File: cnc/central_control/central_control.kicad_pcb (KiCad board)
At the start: 4 copper layers, 103 x 107 mm, 164 parts, among them J1 6pins, J10 Phoenix, J11 3pins, J12 3pins, J13 Screw_Terminal_01x01, J14 3pins, J16 Phoenix, J17 DE9_Socket_MountingHoles, J2 6pins, J20 AVR-UPDI, J3 6pins, J4 7pins, J5 7pins, J6 3pins, J7 3pins, J8 Phoenix, J9 Phoenix, U1 LMR33630ADDA, U10 PC817, U11 PCA9555PW, U12 PCA9555PW, U13 PCA9555PW, U14 PC817, U15 PC817, U16 PC817, U17 PC817, U18 PC817, U19 PC817, U2 LT1785AxS8, U3 ATtiny3226, U5 PC817, U6 PC817, U7 PC817, U8 PC817, U9 PC817

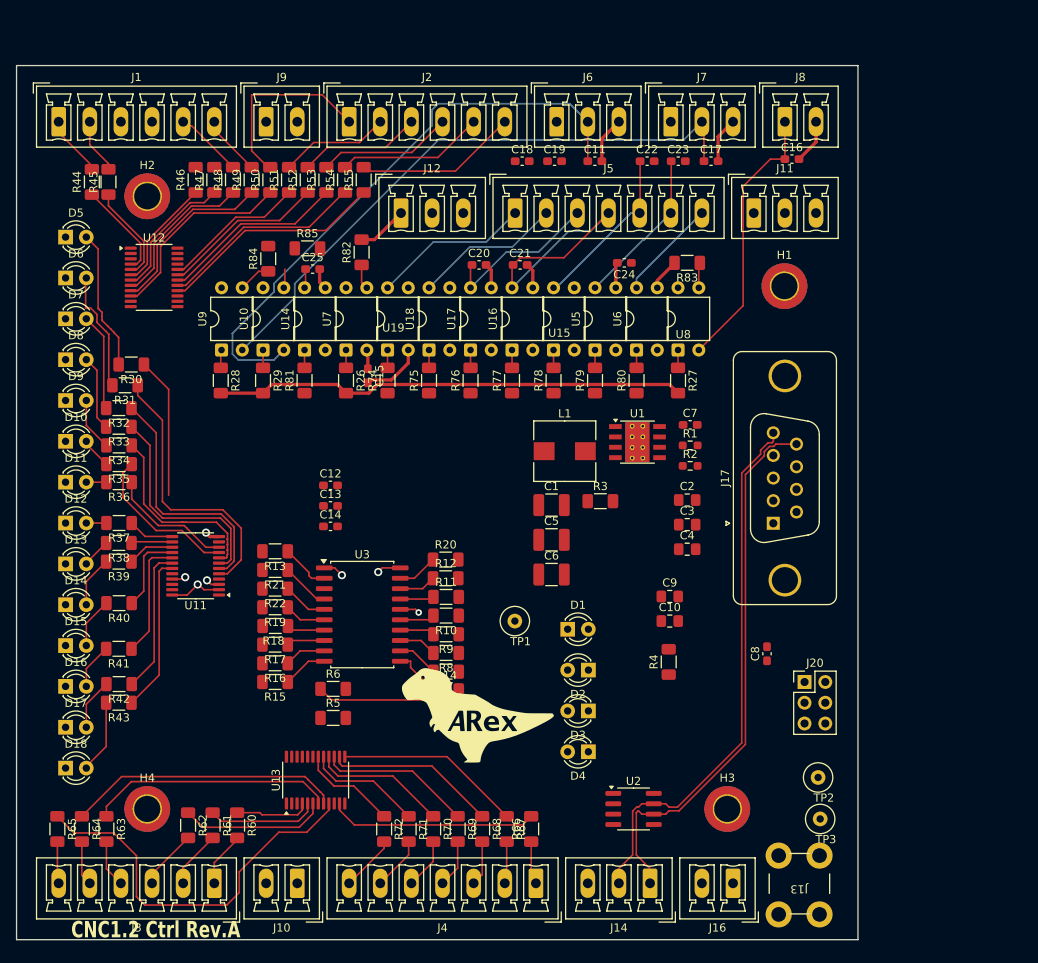
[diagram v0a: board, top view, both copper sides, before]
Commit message: Sent to production
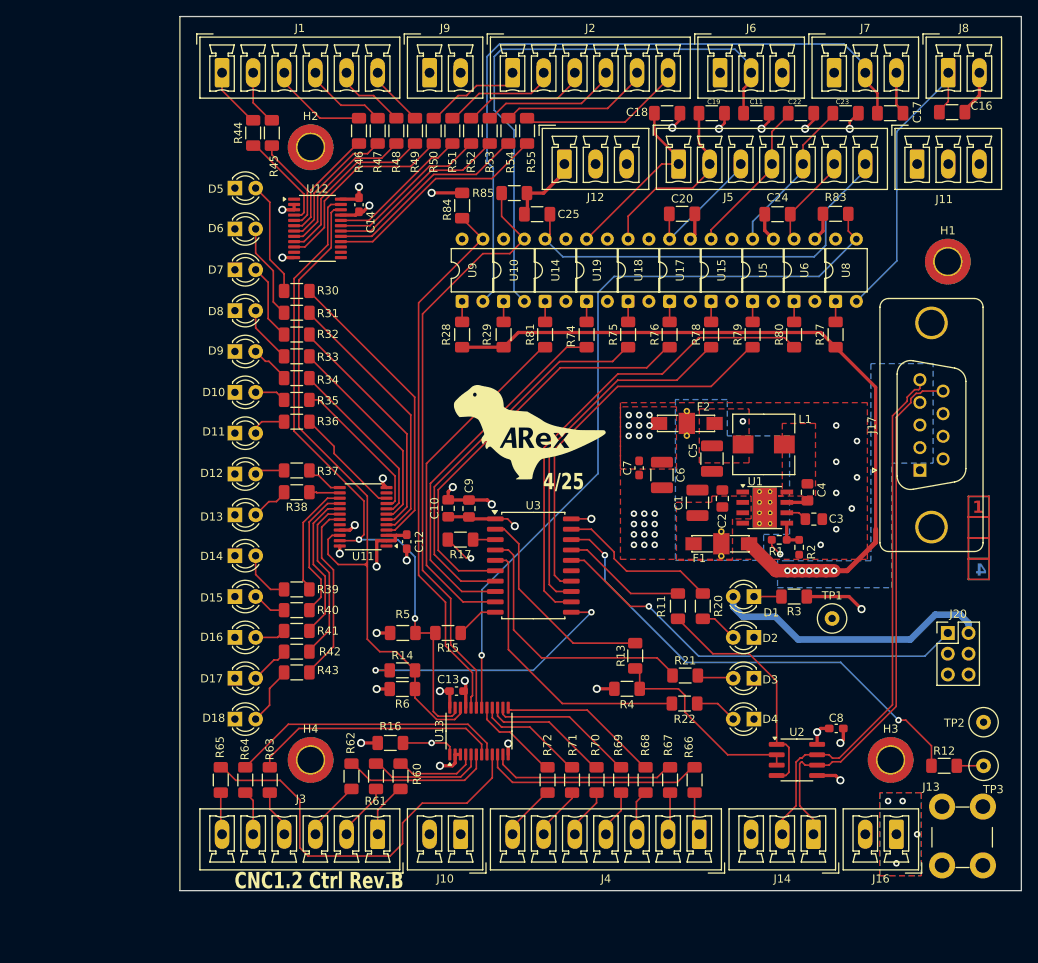
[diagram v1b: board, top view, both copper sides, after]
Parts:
- removed C15, C21: 1nF 250V, Capacitor_SMD:C_0603_1608Metric_Pad1.08x0.95mm_HandSolder
- removed R10, R18, R19, R7, R8, R9: 332, Resistor_SMD:R_1206_3216Metric_Pad1.30x1.75mm_HandSolder
- removed R26: 3k32, Resistor_SMD:R_1206_3216Metric_Pad1.30x1.75mm_HandSolder
- removed R77: 560, Resistor_SMD:R_1206_3216Metric_Pad1.30x1.75mm_HandSolder
- removed R82: 10K, Resistor_SMD:R_1206_3216Metric_Pad1.30x1.75mm_HandSolder
- removed U16, U7: PC817, Package_DIP:DIP-4_W7.62mm
- added F1: ~, adarwoo:Murata_NFM61R, F.Cu at (186.3, 107.5)
- added F2: ~, adarwoo:Murata_NFM61R, F.Cu at (182.1, 92.8)
- C11, C16, C17, C18, C19, C20, C22, C23, C24, C25: footprint Capacitor_SMD:C_0603_1608Metric_Pad1.08x0.95mm_HandSolder -> Capacitor_SMD:C_1206_3216Metric_Pad1.33x1.80mm_HandSolder
- J13: value Screw_Terminal_01x01 -> ~
- R16: value 332 -> 10K
- R27, R28, R29: value 3k32 -> 2k21
- moved R12 65.2 mm to (213.5, 134.7)
- moved R22 52.1 mm to (181.8, 127.1), turned to 0 degrees
- moved R21 51.8 mm to (181.8, 123.7), turned to 0 degrees
- moved R13 45.9 mm to (175.7, 121.3), turned to -90 degrees
- moved C14 39.5 mm to (141.9, 66.0), turned to -90 degrees
- moved TP1 38.8 mm to (199.8, 116.7)
- moved G*** 35.2 mm to (162.8, 93.9)
- moved R20 32.0 mm to (184.0, 115.2), turned to -90 degrees
- moved C10 30.4 mm to (152.8, 103.2), turned to 90 degrees
- moved R28 30.1 mm to (154.5, 81.9)
- moved U14 30.0 mm to (164.7, 77.9)
- moved U9 30.0 mm to (154.5, 77.9)
- moved U10 30.0 mm to (159.6, 77.9)
- moved R81 30.0 mm to (164.7, 81.9)
- moved R29 30.0 mm to (159.6, 81.9)
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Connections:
- net Net-(C5-Pad1) renamed /Power supply/RAW_VCC
- J17 pad 0: unconnected-(J17-PAD-Pad0) -> GND
- J5 pad 4: OC_OUT_LIGHT -> OC_OUT_LASER_CROSS
- J5 pad 5: OC_OUT_LASER_CROSS -> OC_OUT_CAMERA_LIGHT
- J5 pad 6: OC_OUT_CAMERA_LIGHT -> OC_OUT_RELEASE_STEPPERS
- J5 pad 7: OC_OUT_RELEASE_STEPPERS -> OC_OUT_ES
- R16 pad 1: Net-(U3-PB2) -> IO_INT
- R16 pad 2: ISO_IN_SPARE_0 -> VCC
- R17 pad 1: Net-(U3-PB3) -> Net-(U3-PA5)
- R17 pad 2: ISO_IN_SPINDLE_IS_ON -> IO_INT
- R50 pad 1: DOOR_OPEN_CLOSE -> OPEN_CLOSE_DOOR
- R66 pad 2: SPARE_INPUT -> TOUCH_SCREEN_BEEP
- R67 pad 1: TOUCH_SCREEN_BEEP -> SOUNDER
- R68 pad 1: SOUNDER -> LASER_CROSSHAIR
- R69 pad 1: LIGHT_ON_OFF -> CAMERA_LIGHT
- R70 pad 1: LASER_CROSSHAIR -> SPARE_INPUT_1
- R71 pad 1: CAMERA_LIGHT -> SPARE_INPUT_2
- R79 pad 1: ISO_OUT_SPARE_0 -> ISO_OUT_CAMERA_LIGHT
- U11 pad 2: VCC -> GND
- U11 pad 21: GND -> VCC
- U12 pad 1: IO_INT -> unconnected-(U12-~{INT}-Pad1)
- U12 pad 10: DOOR_OPEN_CLOSE -> OPEN_CLOSE_DOOR
- U13 pad 10: unconnected-(U13-IO0_6-Pad10) -> TOUCH_SCREEN_BEEP
- U13 pad 11: SPARE_INPUT -> SOUNDER
- U13 pad 13: TOUCH_SCREEN_BEEP -> LASER_CROSSHAIR
- U13 pad 14: SOUNDER -> CAMERA_LIGHT
- U13 pad 15: LIGHT_ON_OFF -> SPARE_INPUT_1
- U13 pad 16: LASER_CROSSHAIR -> SPARE_INPUT_2
- U13 pad 17: CAMERA_LIGHT -> ~{ES}
- U13 pad 18: ~{ES} -> ISO_IN_SPINDLE_IS_ON
- U13 pad 19: unconnected-(U13-IO1_6-Pad19) -> ISO_IN_DOOR_IS_DOWN
- U13 pad 2: GND -> VCC
- U13 pad 20: unconnected-(U13-IO1_7-Pad20) -> ISO_IN_DOOR_IS_UP
- U13 pad 3: GND -> VCC
- U3 pad 12: Net-(U3-PC0) -> ISO_OUT_RELEASE_STEPPERS
- U3 pad 13: Net-(U3-PC1) -> ISO_OUT_LASER_CROSS
- U3 pad 14: Net-(U3-PC2) -> ISO_OUT_CAMERA_LIGHT
- U3 pad 15: Net-(U3-PC3) -> unconnected-(U3-PC3-Pad15)
- U3 pad 3: unconnected-(U3-PA5-Pad3) -> Net-(U3-PA5)
- U3 pad 6: Net-(U3-PB5) -> ISO_OUT_TOWER_LIGHT_GREEN
- U3 pad 7: Net-(U3-PB4) -> ISO_OUT_TOWER_LIGHT_YELLOW
- U3 pad 8: Net-(U3-PB3) -> ISO_OUT_TOWER_LIGHT_RED
- U3 pad 9: Net-(U3-PB2) -> ISO_OUT_ES
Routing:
- net VCC: track 9.05 -> 139.9 mm, vias 2 -> 20
- net ISO_IN_SPINDLE_IS_ON: track 3.10 -> 94.6 mm, vias 0 -> 1
- net SDA: track 0.00 -> 83.3 mm, vias 0 -> 2
- net ISO_IN_DOOR_IS_DOWN: track 2.34 -> 74.0 mm
- net SCL: track 18.0 -> 86.6 mm
- net ISO_IN_DOOR_IS_UP: track 4.01 -> 67.1 mm
- net ISO_OUT_RELEASE_STEPPERS: track 0.00 -> 58.1 mm
- net Net-(U3-PA2): track 4.54 -> 58.8 mm, vias 0 -> 2
- net ISO_OUT_TOWER_LIGHT_GREEN: track 0.00 -> 51.0 mm
- net UPDI: track 2.41 -> 52.1 mm
- net OC_OUT_ES: track 2.34 -> 51.1 mm
- net ISO_OUT_TOWER_LIGHT_YELLOW: track 0.00 -> 47.9 mm
- net ISO_OUT_CAMERA_LIGHT: track 0.00 -> 47.2 mm
- net ISO_OUT_LASER_CROSS: track 0.00 -> 45.6 mm
- net ISO_OUT_TOWER_LIGHT_RED: track 0.00 -> 45.3 mm
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- added copper zone on B.Cu, net +24V
- added copper zone on F.Cu, net +24V
- added copper zone on F.Cu, net /Power supply/RAW_VCC
- added copper zone on B.Cu, net GND
- added copper zone on F.Cu, net GND
- added copper zone on F.Cu, net Net-(U1-SW)
- added copper zone on F.Cu, net VCC
- added copper zone on F.Cu, net VDD
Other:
- board text added: "1"
- board text added: "2"
- board text added: "3"
- board text added: "4"
- board text added: "4/25"
- board text added: "CNC1.2 Ctrl Rev.B"
- board text removed: "CNC1.2 Ctrl Rev.A"
